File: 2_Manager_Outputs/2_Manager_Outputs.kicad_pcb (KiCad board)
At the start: 2 copper layers, 100 x 100 mm, 48 parts, among them J1 VDD 12V, J11 I2C, J2 RS232, J3 VDD 5V, J4 SPEAKER, J5 RESET, P3 SPI, SW1 Reset, U1 ATMEGA328P-AU_MIO, U4 LD1117S33TR_MIO, Y1 Crystal

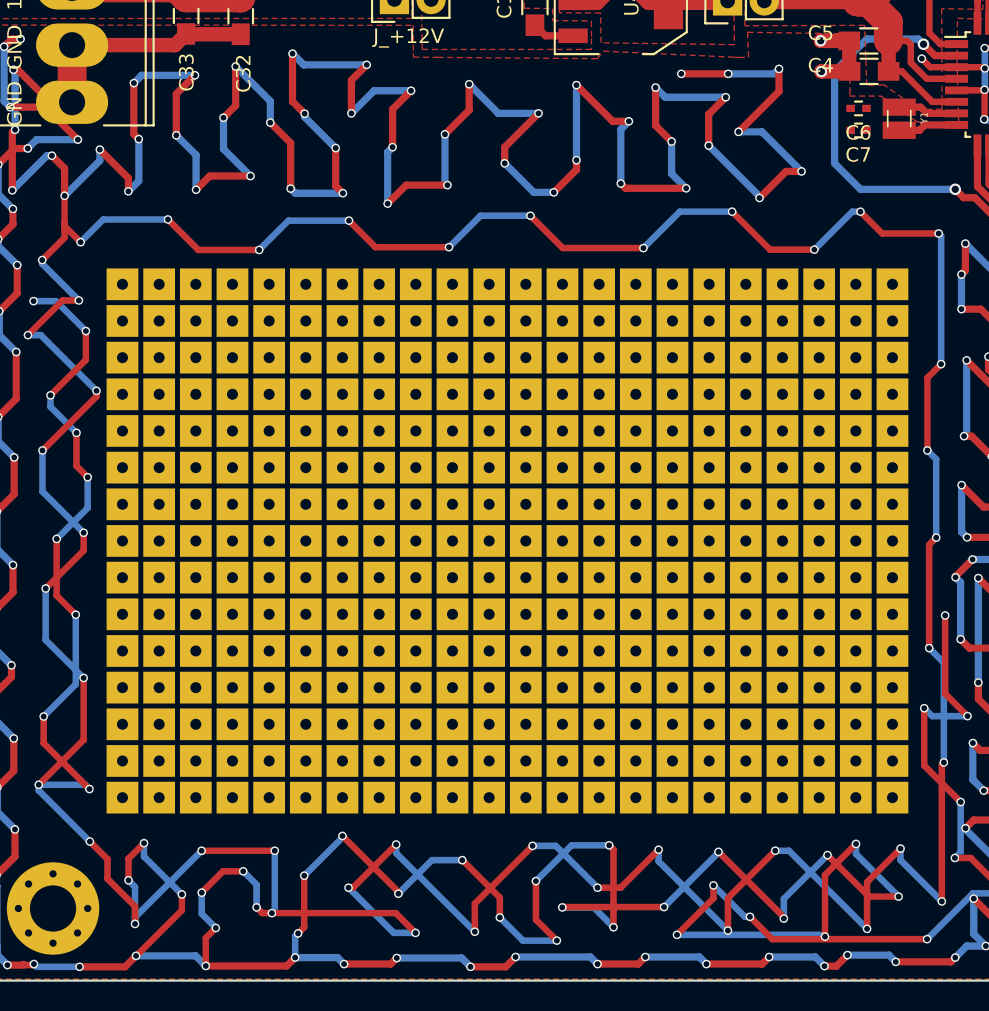
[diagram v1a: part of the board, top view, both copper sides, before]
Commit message: Revert "//"
This reverts commit a491b2ffacc572f737e67cceefcc72cf1d6daf07.
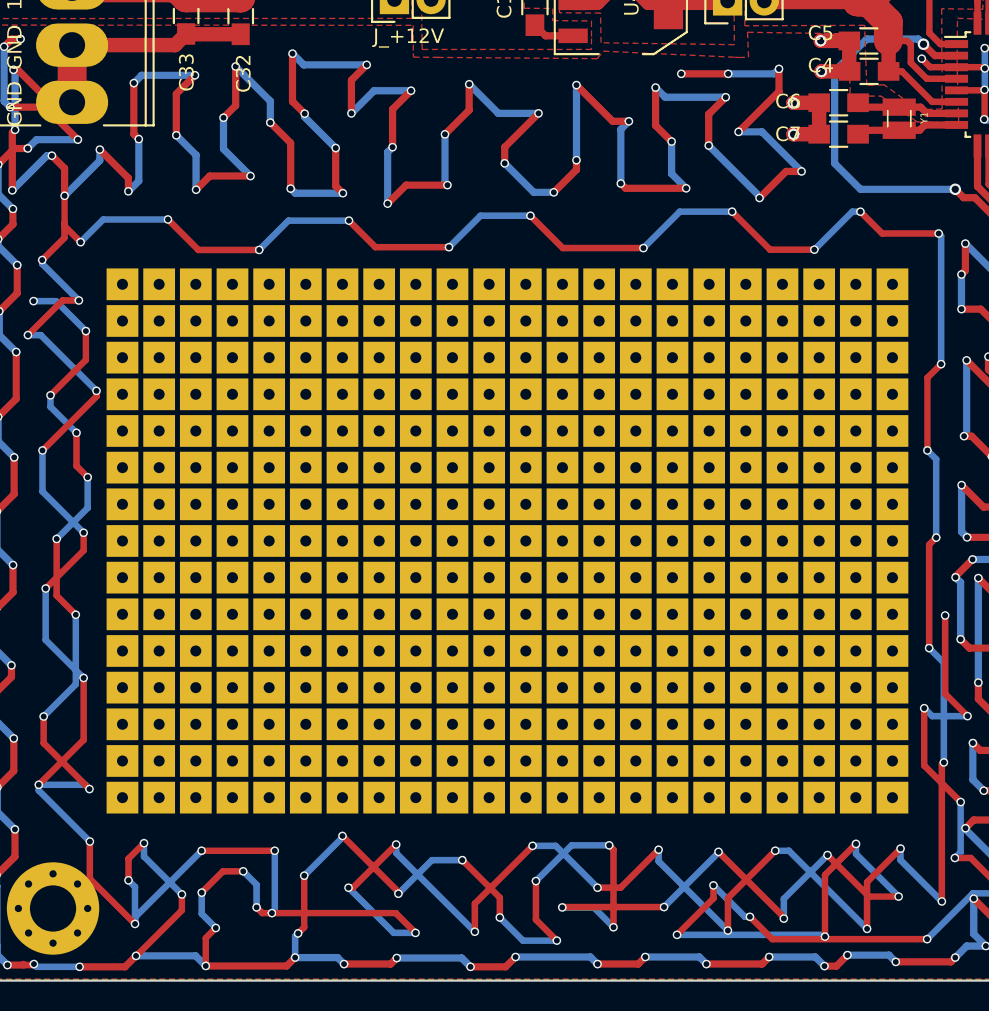
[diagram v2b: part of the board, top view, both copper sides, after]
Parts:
- C6, C7: footprint Capacitors_SMD:C_0402 -> Resistors_SMD:R_0805_HandSoldering
- moved C6 1.44 mm to (139.4, 61.2)
- moved C7 1.40 mm to (139.4, 63.4)
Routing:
- net /GND: track 2266.8 -> 2272.7 mm, vias 564 -> 566
- net /XTAL1: track 4.15 -> 7.13 mm
- net /XTAL2: track 4.12 -> 7.09 mm
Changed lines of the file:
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@@
   (general
     (links 136)
-    (no_connects 4)
-    (area 79.924999 21.924999 180.075001 122.075001)
+    (no_connects 0)
+    (area 72.177143 20.77592 187.822858 123.045)
     (thickness 1.6)
     (drawings 5)
-    (tracks 2111)
+    (tracks 2122)
     (zones 0)
     (modules 48)
@@
   )
   (module Resistors_SMD:R_0805_HandSoldering (layer F.Cu)
+    (at 139.42 61.18 180)
+    (descr "Resistor SMD 0805, hand soldering")
+    (tags "resistor 0805")
+    (attr smd)
+    (fp_text reference C6 (at 3.49 0.08 180) (layer F.SilkS)
+      (effects (font (size 1 1) (thickness 0.15)))
+    )
+    (fp_text value 8pF (at 0 2.1 180) (layer F.Fab)
+      (effects (font (size 1 1) (thickness 0.15)))
+    )
+    (fp_line (start -2.4 -1) (end 2.4 -1) (layer F.CrtYd) (width 0.05))
+    (fp_line (start -2.4 1) (end 2.4 1) (layer F.CrtYd) (width 0.05))
+    (fp_line (start -2.4 -1) (end -2.4 1) (layer F.CrtYd) (width 0.05))
+    (fp_line (start 2.4 -1) (end 2.4 1) (layer F.CrtYd) (width 0.05))
+    (fp_line (start 0.6 0.875) (end -0.6 0.875) (layer F.SilkS) (width 0.15))
+    (fp_line (start -0.6 -0.875) (end 0.6 -0.875) (layer F.SilkS) (width 0.15))
+    (pad 1 smd rect (at -1.35 0 180) (size 1.5 1.3) (layers F.Cu F.Paste F.Mask)
+      (net 28 /XTAL1))
+    (pad 2 smd rect (at 1.35 0 180) (size 1.5 1.3) (layers F.Cu F.Paste F.Mask)
+      (net 1 /GND))
+    (model Resistors_SMD.3dshapes/R_0805_HandSoldering.wrl
+      (at (xyz 0 0 0))
+      (scale (xyz 1 1 1))
+      (rotate (xyz 0 0 0))
+    )
+  )
+  (module Resistors_SMD:R_0805_HandSoldering (layer F.Cu)
+    (at 139.42 63.36 180)
+    (descr "Resistor SMD 0805, hand soldering")
+    (tags "resistor 0805")
+    (attr smd)
+    (fp_text reference C7 (at 3.49 -0.01 180) (layer F.SilkS)
+      (effects (font (size 1 1) (thickness 0.15)))
+    )
+    (fp_text value 8pF (at 0 2.1 180) (layer F.Fab)
+      (effects (font (size 1 1) (thickness 0.15)))
+    )
+    (fp_line (start -2.4 -1) (end 2.4 -1) (layer F.CrtYd) (width 0.05))
+    (fp_line (start -2.4 1) (end 2.4 1) (layer F.CrtYd) (width 0.05))
+    (fp_line (start -2.4 -1) (end -2.4 1) (layer F.CrtYd) (width 0.05))
+    (fp_line (start 2.4 -1) (end 2.4 1) (layer F.CrtYd) (width 0.05))
+    (fp_line (start 0.6 0.875) (end -0.6 0.875) (layer F.SilkS) (width 0.15))
+    (fp_line (start -0.6 -0.875) (end 0.6 -0.875) (layer F.SilkS) (width 0.15))
+    (pad 1 smd rect (at -1.35 0 180) (size 1.5 1.3) (layers F.Cu F.Paste F.Mask)
+      (net 29 /XTAL2))
+    (pad 2 smd rect (at 1.35 0 180) (size 1.5 1.3) (layers F.Cu F.Paste F.Mask)
+      (net 1 /GND))
+    (model Resistors_SMD.3dshapes/R_0805_HandSoldering.wrl
+      (at (xyz 0 0 0))
+      (scale (xyz 1 1 1))
+      (rotate (xyz 0 0 0))
+    )
+  )
+  (module Resistors_SMD:R_0805_HandSoldering (layer F.Cu)
     (at 133.61 46.91 270)
     (descr "Resistor SMD 0805, hand soldering")
@@
     )
   )
-  (module Capacitors_SMD:C_0402 (layer F.Cu)
-    (at 140.8 61.575 180)
-    (descr "Capacitor SMD 0402, reflow soldering, AVX (see smccp.pdf)")
-    (tags "capacitor 0402")
-    (attr smd)
-    (fp_text reference C6 (at 0 -1.7 180) (layer F.SilkS)
-      (effects (font (size 1 1) (thickness 0.15)))
-    )
-    (fp_text value 8pF (at 0 1.7 180) (layer F.Fab)
-      (effects (font (size 1 1) (thickness 0.15)))
-    )
-    (fp_line (start -1.15 -0.6) (end 1.15 -0.6) (layer F.CrtYd) (width 0.05))
-    (fp_line (start -1.15 0.6) (end 1.15 0.6) (layer F.CrtYd) (width 0.05))
-    (fp_line (start -1.15 -0.6) (end -1.15 0.6) (layer F.CrtYd) (width 0.05))
-    (fp_line (start 1.15 -0.6) (end 1.15 0.6) (layer F.CrtYd) (width 0.05))
-    (fp_line (start 0.25 -0.475) (end -0.25 -0.475) (layer F.SilkS) (width 0.15))
-    (fp_line (start -0.25 0.475) (end 0.25 0.475) (layer F.SilkS) (width 0.15))
-    (pad 1 smd rect (at -0.55 0 180) (size 0.6 0.5) (layers F.Cu F.Paste F.Mask)
-      (net 28 /XTAL1))
-    (pad 2 smd rect (at 0.55 0 180) (size 0.6 0.5) (layers F.Cu F.Paste F.Mask)
-      (net 1 /GND))
-    (model Capacitors_SMD.3dshapes/C_0402.wrl
-      (at (xyz 0 0 0))
-      (scale (xyz 1 1 1))
-      (rotate (xyz 0 0 0))
-    )
-  )
-  (module Capacitors_SMD:C_0402 (layer F.Cu)
-    (at 140.8 63.1 180)
-    (descr "Capacitor SMD 0402, reflow soldering, AVX (see smccp.pdf)")
-    (tags "capacitor 0402")
-    (attr smd)
-    (fp_text reference C7 (at 0 -1.7 180) (layer F.SilkS)
-      (effects (font (size 1 1) (thickness 0.15)))
-    )
-    (fp_text value 8pF (at 0 1.7 180) (layer F.Fab)
-      (effects (font (size 1 1) (thickness 0.15)))
-    )
-    (fp_line (start -1.15 -0.6) (end 1.15 -0.6) (layer F.CrtYd) (width 0.05))
-    (fp_line (start -1.15 0.6) (end 1.15 0.6) (layer F.CrtYd) (width 0.05))
-    (fp_line (start -1.15 -0.6) (end -1.15 0.6) (layer F.CrtYd) (width 0.05))
-    (fp_line (start 1.15 -0.6) (end 1.15 0.6) (layer F.CrtYd) (width 0.05))
-    (fp_line (start 0.25 -0.475) (end -0.25 -0.475) (layer F.SilkS) (width 0.15))
-    (fp_line (start -0.25 0.475) (end 0.25 0.475) (layer F.SilkS) (width 0.15))
-    (pad 1 smd rect (at -0.55 0 180) (size 0.6 0.5) (layers F.Cu F.Paste F.Mask)
-      (net 29 /XTAL2))
-    (pad 2 smd rect (at 0.55 0 180) (size 0.6 0.5) (layers F.Cu F.Paste F.Mask)
-      (net 1 /GND))
-    (model Capacitors_SMD.3dshapes/C_0402.wrl
-      (at (xyz 0 0 0))
-      (scale (xyz 1 1 1))
-      (rotate (xyz 0 0 0))
-    )
-  )
   (module Pin_Headers:Pin_Header_Straight_1x02 (layer F.Cu)
     (at 94.3 27.275 270)
@@
   (segment (start 175.3 24.31) (end 176.17 24.31) (width 0.5) (layer F.Cu) (net 0))
   (segment (start 172.59 25.91) (end 173.7 25.91) (width 0.5) (layer B.Cu) (net 0))
-  (segment (start 90.68 118.07) (end 90.68 116.855) (width 0.45) (layer F.Cu) (net 1))
-  (segment (start 88.775 113.585) (end 87.55 112.36) (width 0.45) (layer F.Cu) (net 1))
-  (segment (start 88.775 114.95) (end 88.775 113.585) (width 0.45) (layer F.Cu) (net 1))
-  (segment (start 90.68 116.855) (end 88.775 114.95) (width 0.45) (layer F.Cu) (net 1))
   (segment (start 85.425 36.575) (end 86.9 36.575) (width 0.5) (layer F.Cu) (net 1))
   (via (at 86.925 36.6) (size 0.6) (drill 0.4) (layers F.Cu B.Cu) (net 1))
@@
   (via (at 90.68 118.07) (size 0.6) (drill 0.4) (layers F.Cu B.Cu) (net 1))
   (segment (start 85.79 70.54) (end 85.79 69.52) (width 0.45) (layer F.Cu) (net 1))
+  (segment (start 90.68 118.07) (end 87.55 114.94) (width 0.45) (layer F.Cu) (net 1))
+  (segment (start 87.55 114.94) (end 87.55 112.36) (width 0.45) (layer F.Cu) (net 1))
   (via (at 87.55 112.36) (size 0.6) (drill 0.4) (layers F.Cu B.Cu) (net 1))
   (segment (start 87.55 112.36) (end 84.01 108.82) (width 0.45) (layer B.Cu) (net 1))
@@
   (segment (start 145.77 58.72) (end 145.18 58.13) (width 0.45) (layer F.Cu) (net 1))
   (via (at 145.18 58.13) (size 0.6) (drill 0.4) (layers F.Cu B.Cu) (net 1))
+  (segment (start 138.07 63.36) (end 136.31 63.36) (width 1) (layer F.Cu) (net 1))
+  (segment (start 136.3 63.37) (end 136.29 63.37) (width 1) (layer B.Cu) (net 1))
+  (via (at 136.3 63.37) (size 0.8) (drill 0.5) (layers F.Cu B.Cu) (net 1))
+  (segment (start 136.31 63.36) (end 136.3 63.37) (width 1) (layer F.Cu) (net 1))
+  (segment (start 138.07 61.18) (end 136.3 61.18) (width 1) (layer F.Cu) (net 1))
+  (via (at 136.28 61.2) (size 0.8) (drill 0.5) (layers F.Cu B.Cu) (net 1))
+  (segment (start 136.3 61.18) (end 136.28 61.2) (width 1) (layer F.Cu) (net 1))
   (segment (start 140.18 59.01) (end 138.24 59.01) (width 1) (layer F.Cu) (net 1))
   (via (at 138.23 59.02) (size 0.8) (drill 0.5) (layers F.Cu B.Cu) (net 1))
@@
   (via (at 138.18 56.89) (size 0.8) (drill 0.5) (layers F.Cu B.Cu) (net 1))
   (segment (start 138.19 56.9) (end 138.18 56.89) (width 1) (layer F.Cu) (net 1))
+  (segment (start 138.07 61.18) (end 138.07 63.36) (width 1) (layer F.Cu) (net 1))
+  (segment (start 138.07 61.18) (end 138.07 61.12) (width 1) (layer F.Cu) (net 1))
   (segment (start 140.16 56.9) (end 140.16 58.99) (width 1) (layer F.Cu) (net 1))
   (segment (start 140.16 58.99) (end 140.18 59.01) (width 1) (layer F.Cu) (net 1))
@@
   (segment (start 123.8 51.82) (end 123.8 49.56) (width 1) (layer F.Cu) (net 27))
   (segment (start 122.7 54.26) (end 123.8 53.16) (width 1) (layer F.Cu) (net 27))
+  (segment (start 143.62 61.49) (end 141.08 61.49) (width 0.5) (layer F.Cu) (net 28))
+  (segment (start 141.08 61.49) (end 140.77 61.18) (width 0.5) (layer F.Cu) (net 28))
   (segment (start 143.62 61.49) (end 145.11 61.49) (width 0.5) (layer F.Cu) (net 28))
   (segment (start 145.54 61.92) (end 147.59 61.92) (width 0.5) (layer F.Cu) (net 28))
   (segment (start 145.11 61.49) (end 145.54 61.92) (width 0.5) (layer F.Cu) (net 28))
+  (segment (start 143.62 63.09) (end 141.04 63.09) (width 0.5) (layer F.Cu) (net 29))
+  (segment (start 141.04 63.09) (end 140.77 63.36) (width 0.5) (layer F.Cu) (net 29))
   (segment (start 143.62 63.09) (end 145.03 63.09) (width 0.5) (layer F.Cu) (net 29))
   (segment (start 145.4 62.72) (end 147.59 62.72) (width 0.5) (layer F.Cu) (net 29))
